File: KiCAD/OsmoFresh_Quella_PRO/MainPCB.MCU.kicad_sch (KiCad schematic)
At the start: 25 parts, among them CN11 Conn_01x04_Pin, CN14 Conn_01x02_Pin, CN2 Conn_01x02_Pin, CN6 Conn_01x02_Pin, CN7 Conn_01x02_Pin, CN9 Conn_01x02_Pin

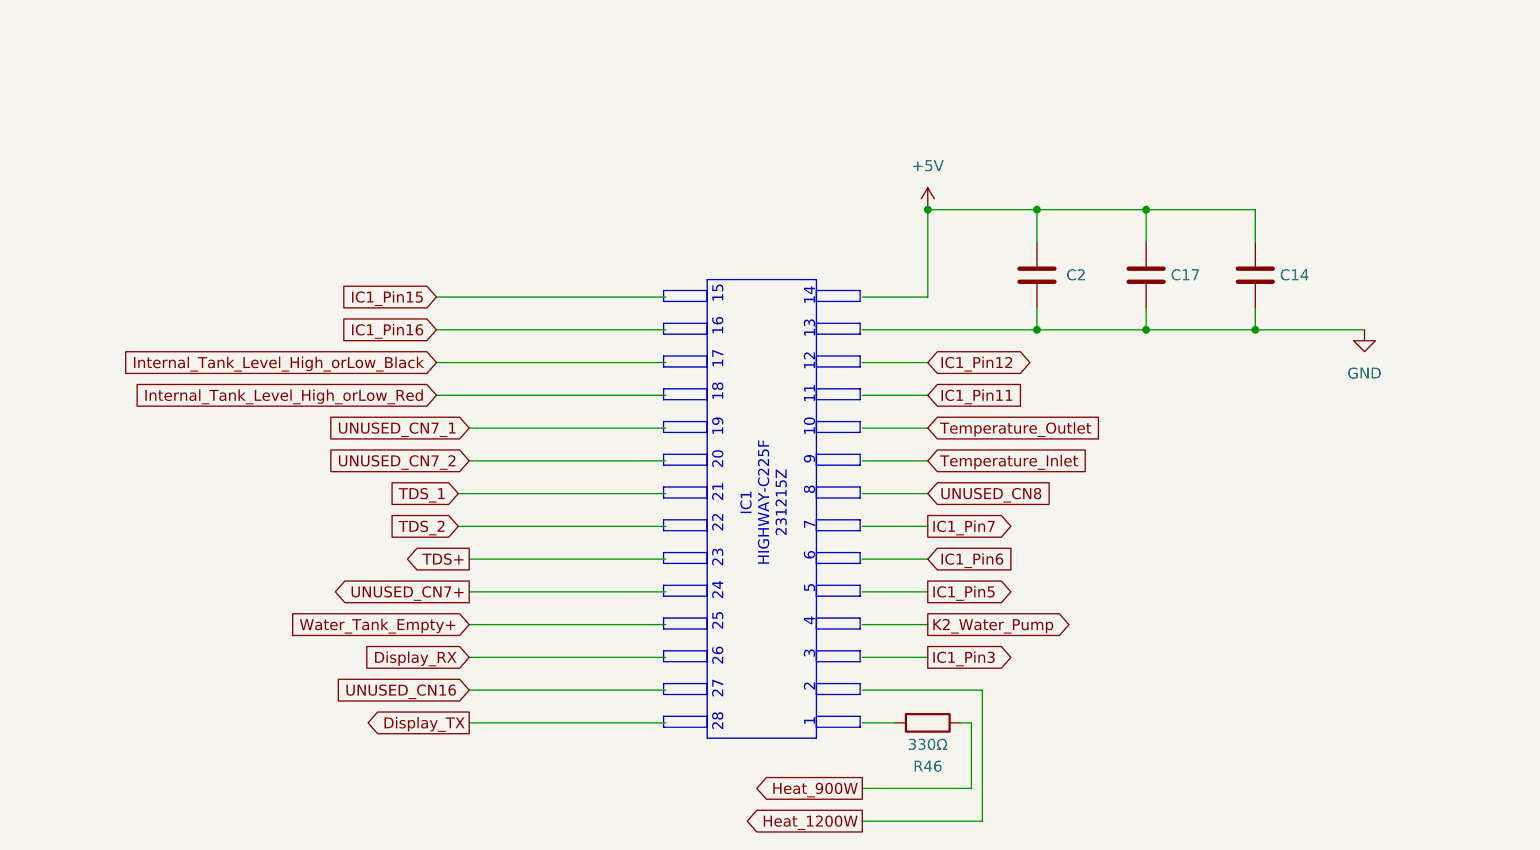
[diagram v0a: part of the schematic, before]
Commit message: Update Schematics
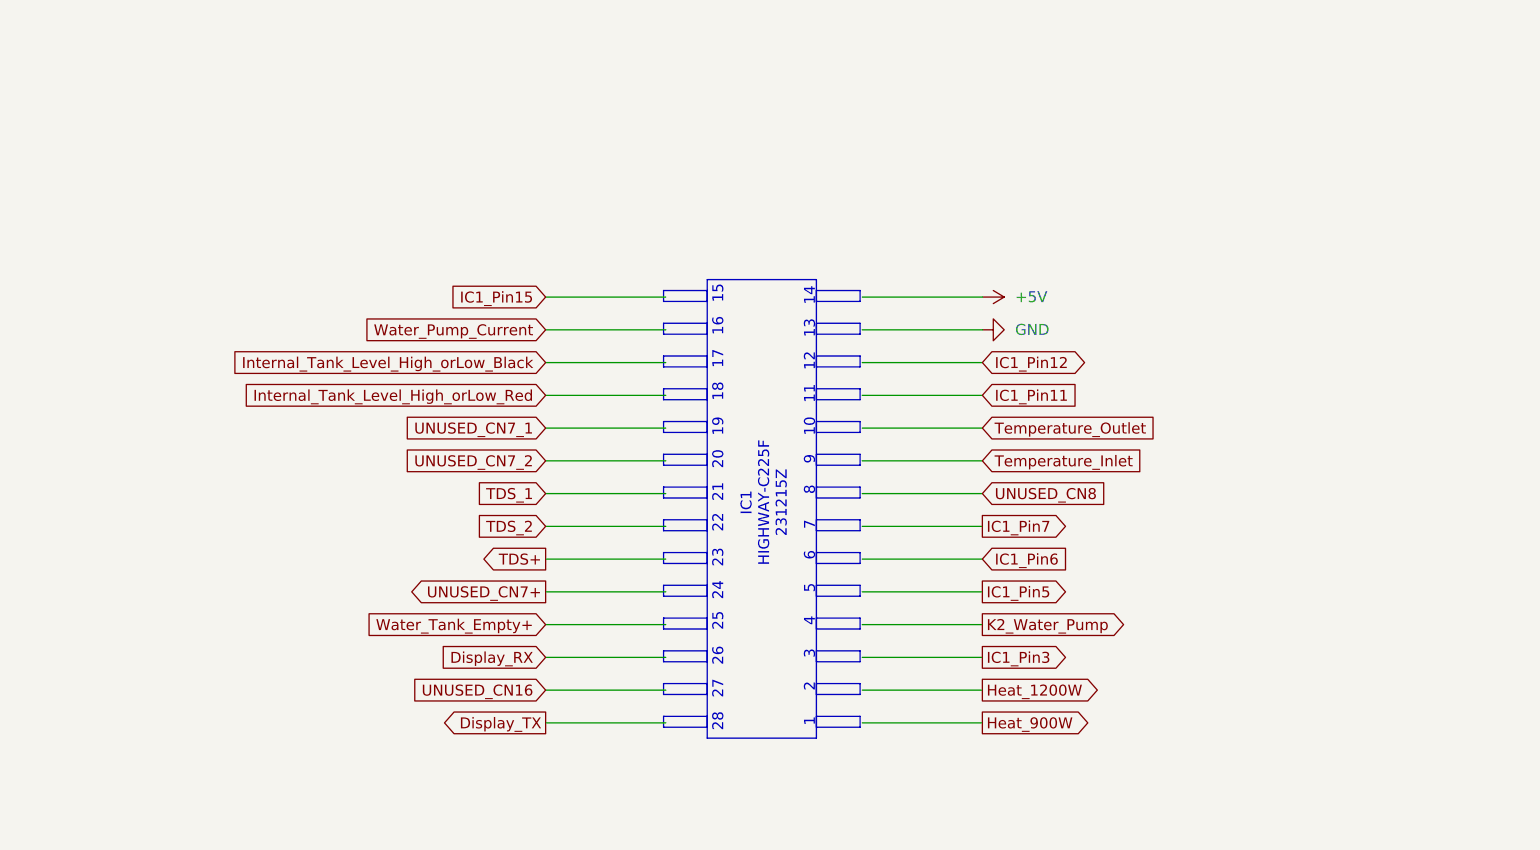
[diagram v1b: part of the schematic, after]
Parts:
- removed C14, C17, C2: unkown, symbol Device:C
- removed R46: 330Ω, symbol Device:R
